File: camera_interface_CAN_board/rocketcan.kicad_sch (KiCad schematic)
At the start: 11 parts, among them J2 G125-MH104M4-04AD000P, U2 canhw:MCP2562, U4 INA180A1

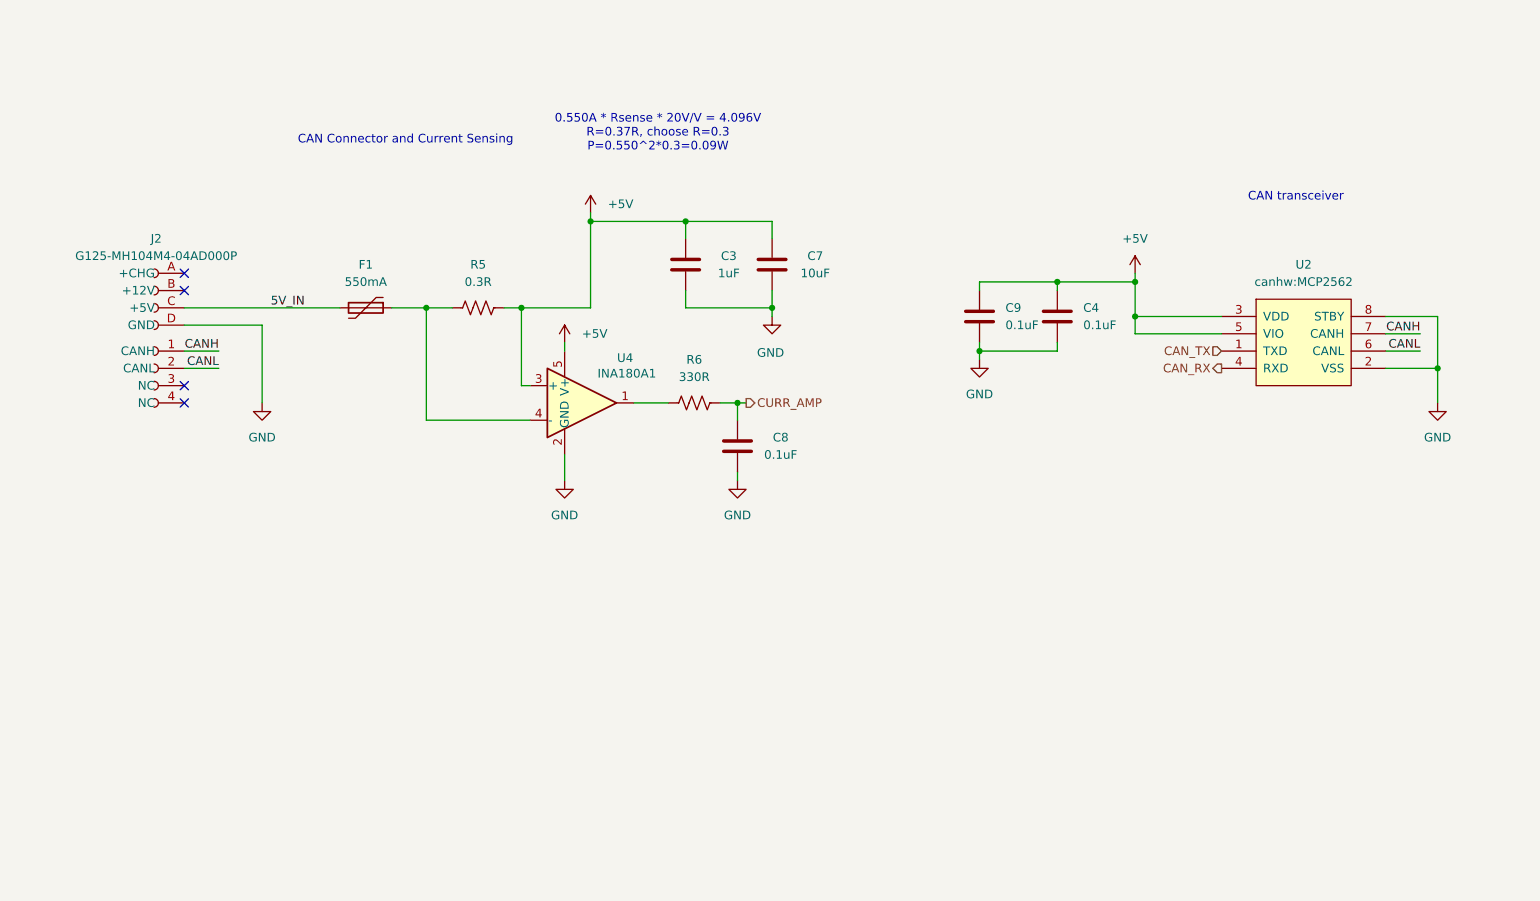
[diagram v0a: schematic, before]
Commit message: ready for review
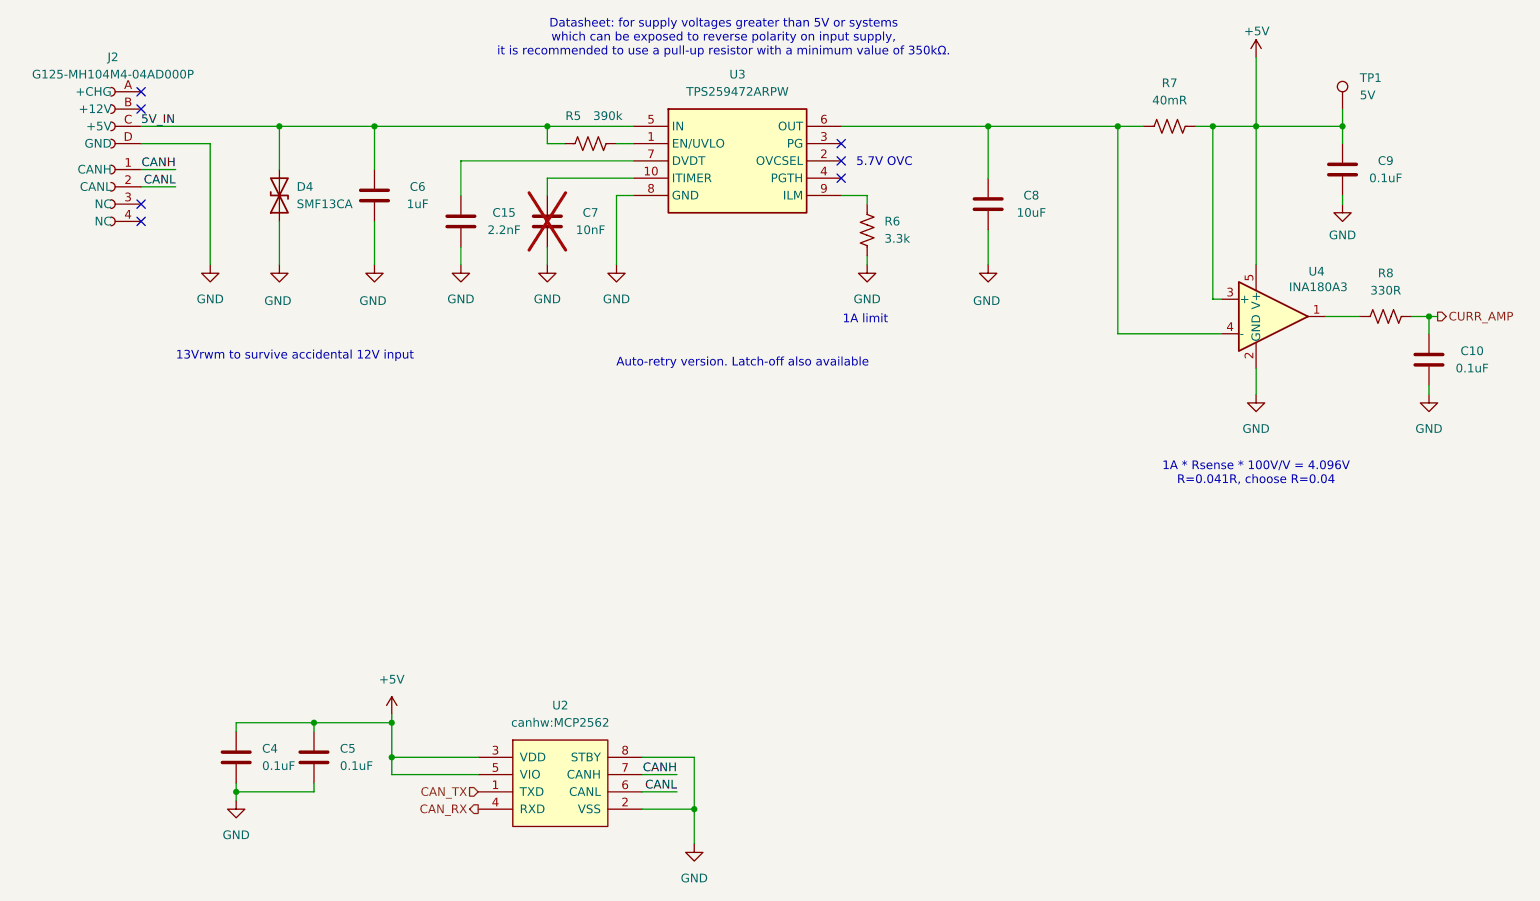
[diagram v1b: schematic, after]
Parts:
- removed C3: 1uF, Capacitor_SMD:C_0603_1608Metric_Pad1.08x0.95mm_HandSolder, symbol Device:C
- removed F1: 550mA, Fuse:Fuse_0805_2012Metric_Pad1.15x1.40mm_HandSolder, symbol Device:Polyfuse
- added C15: 2.2nF, Capacitor_SMD:C_0603_1608Metric_Pad1.08x0.95mm_HandSolder, symbol Device:C
- added C6: 1uF, Capacitor_SMD:C_0603_1608Metric_Pad1.08x0.95mm_HandSolder, symbol Device:C
- added C8: 10uF, Capacitor_SMD:C_0805_2012Metric_Pad1.18x1.45mm_HandSolder, symbol Device:C
- added C9: 0.1uF, Capacitor_SMD:C_0603_1608Metric_Pad1.08x0.95mm_HandSolder, symbol Device:C
- added D4: SMF13CA, Diode_SMD:D_SMF, symbol Device:D_TVS
- added R5: 390k, Resistor_SMD:R_0603_1608Metric_Pad0.98x0.95mm_HandSolder, symbol Device:R_US
- added R6: 3.3k, Resistor_SMD:R_0603_1608Metric_Pad0.98x0.95mm_HandSolder, symbol Device:R_US
- added TP1: 5V, TestPoint:TestPoint_Pad_D1.0mm, symbol Connector:TestPoint
- added U3: TPS259472ARPW, canhw_footprints:TPS25947xx, symbol canhw:TPS259472ARPW
- C7: value 10uF -> 10nF; footprint Capacitor_SMD:C_0805_2012Metric_Pad1.18x1.45mm_HandSolder -> Capacitor_SMD:C_0603_1608Metric_Pad1.08x0.95mm_HandSolder; now not fitted
- R7: renamed from R5; value 0.3R -> 40mR; footprint Resistor_SMD:R_0603_1608Metric_Pad0.98x0.95mm_HandSolder -> Resistor_SMD:R_0805_2012Metric_Pad1.20x1.40mm_HandSolder
- U4: value INA180A1 -> INA180A3
- renumbered C8 to C10, C9 to C4, C4 to C5, R6 to R8
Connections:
- net +5V: now also C9.2, TP1.1; no longer C7.2
- net 5V_IN: now also C6.2, D4.2 (A2), R5.1, U3.5 (IN)
- net GND: now also C15.1, C6.1, C8.1, C9.1, D4.1 (A1), R6.2, U3.8 (GND)
- net at R7.2, U4.4 (-): now also C8.2, U3.6 (OUT)
- new net: R6.1, U3.9 (ILM)
- new net: R5.2, U3.1 (EN/UVLO)
- new net: C7.2, U3.10 (ITIMER)
- new net: C15.2, U3.7 (DVDT)
- no-connect marks 4 -> 7
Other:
- note added: "13Vrwm to survive accidental 12V input"
- note added: "1A * Rsense * 100V/V = 4.096V R=0.041R, choose R=0.04"
- note added: "1A limit"
- note added: "5.7V OVC"
- note added: "Auto-retry version. Latch-off also available"
- note added: "Datasheet: for supply voltages greater than 5V or systems which can be exposed to reverse polarity on input supply, it is recommended to use a pull-up resistor with a minimum value of 350kΩ."
- note removed: "0.550A * Rsense * 20V/V = 4.096V R=0.37R, choose R=0.3 P=0.550^2*0.3=0.09W"
- note removed: "CAN Connector and Current Sensing"
- note removed: "CAN transceiver"
- company: (none) -> Waterloo Rocketry
- title: (none) -> Camera Interface Board
- moved on the sheet: C10, C4, C5, J2, R7, R8, U2, U4

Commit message: schematic
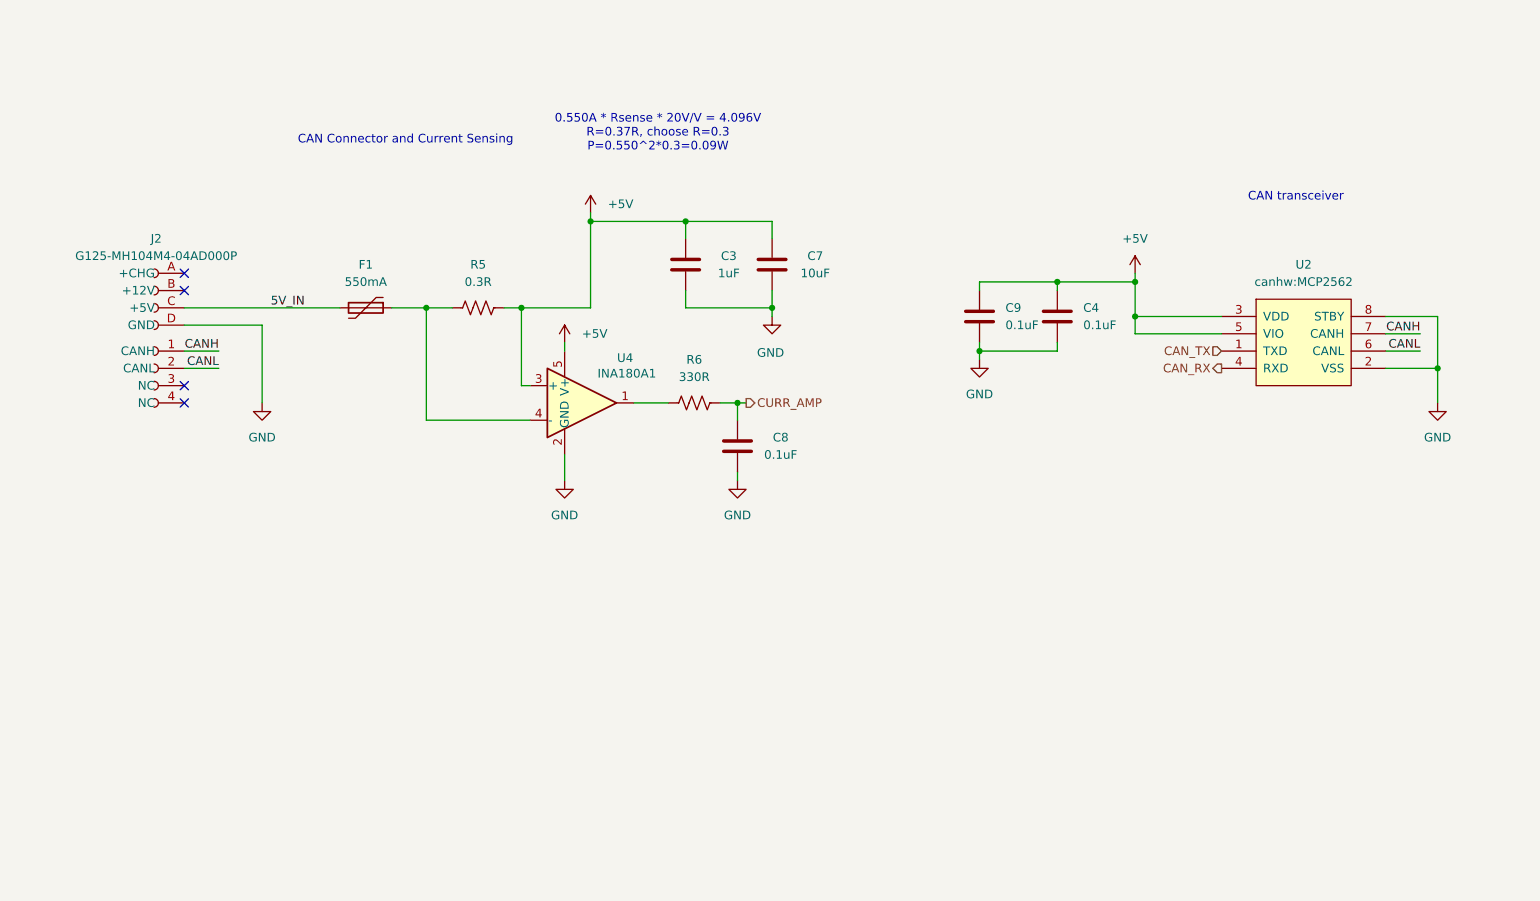
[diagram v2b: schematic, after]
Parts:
- removed C15: 2.2nF, Capacitor_SMD:C_0603_1608Metric_Pad1.08x0.95mm_HandSolder, symbol Device:C
- removed C6: 1uF, Capacitor_SMD:C_0603_1608Metric_Pad1.08x0.95mm_HandSolder, symbol Device:C
- removed C8: 10uF, Capacitor_SMD:C_0805_2012Metric_Pad1.18x1.45mm_HandSolder, symbol Device:C
- removed C9: 0.1uF, Capacitor_SMD:C_0603_1608Metric_Pad1.08x0.95mm_HandSolder, symbol Device:C
- removed D4: SMF13CA, Diode_SMD:D_SMF, symbol Device:D_TVS
- removed R5: 390k, Resistor_SMD:R_0603_1608Metric_Pad0.98x0.95mm_HandSolder, symbol Device:R_US
- removed R6: 3.3k, Resistor_SMD:R_0603_1608Metric_Pad0.98x0.95mm_HandSolder, symbol Device:R_US
- removed TP1: 5V, TestPoint:TestPoint_Pad_D1.0mm, symbol Connector:TestPoint
- removed U3: TPS259472ARPW, canhw_footprints:TPS25947xx, symbol canhw:TPS259472ARPW
- added C3: 1uF, Capacitor_SMD:C_0603_1608Metric_Pad1.08x0.95mm_HandSolder, symbol Device:C
- added F1: 550mA, Fuse:Fuse_0805_2012Metric_Pad1.15x1.40mm_HandSolder, symbol Device:Polyfuse
- C7: value 10nF -> 10uF; footprint Capacitor_SMD:C_0603_1608Metric_Pad1.08x0.95mm_HandSolder -> Capacitor_SMD:C_0805_2012Metric_Pad1.18x1.45mm_HandSolder; now fitted
- R5: renamed from R7; value 40mR -> 0.3R; footprint Resistor_SMD:R_0805_2012Metric_Pad1.20x1.40mm_HandSolder -> Resistor_SMD:R_0603_1608Metric_Pad0.98x0.95mm_HandSolder
- U4: value INA180A3 -> INA180A1
- renumbered C5 to C4, C10 to C8, C4 to C9, R8 to R6
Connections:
- net +5V: now also C7.2, C3.2
- net 5V_IN: now also F1.2
- net GND: now also C3.1
- net at R5.2, U4.4 (-): now also F1.1
- no-connect marks 7 -> 4
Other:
- note added: "0.550A * Rsense * 20V/V = 4.096V R=0.37R, choose R=0.3 P=0.550^2*0.3=0.09W"
- note added: "CAN Connector and Current Sensing"
- note added: "CAN transceiver"
- note removed: "13Vrwm to survive accidental 12V input"
- note removed: "1A * Rsense * 100V/V = 4.096V R=0.041R, choose R=0.04"
- note removed: "1A limit"
- note removed: "5.7V OVC"
- note removed: "Auto-retry version. Latch-off also available"
- note removed: "Datasheet: for supply voltages greater than 5V or systems which can be exposed to reverse polarity on input supply, it is recommended to use a pull-up resistor with a minimum value of 350kΩ."
- company: Waterloo Rocketry -> (none)
- title: Camera Interface Board -> (none)
- moved on the sheet: C4, C8, C9, J2, R5, R6, U2, U4
